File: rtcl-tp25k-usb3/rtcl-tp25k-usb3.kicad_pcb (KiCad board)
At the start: 4 copper layers, 80 x 35 mm, 109 parts, among them J1 ZX360D-B-10P(30), J10 SSQ-106-02-F-D-RA, J2 CF20221V0R0-NH, J3 DF40C(2.0)-60DS-0.4V(51), J4 DF40C(2.0)-60DS-0.4V(51), J5 JTAG, J6 Conn_01x02, J7 Conn_01x03, Q2 NTK3134NT1G, Q3 NTK3134NT1G, Q4 NTK3134NT1G, Q5 NTK3134NT1G, Q6 NTK3134NT1G, SW1 B3U-1100P, SW2 B3U-1100P, SW3 218-2LPSTR, SW4 B3U-1100P, U1 FT601Q, U2 TPD4E05U06DQA, U3 USBLC6-2P6, U4 TPS62826DMQR, U5 PCA9306DC, X1 ABM8-30.000MHZ-D1X-T

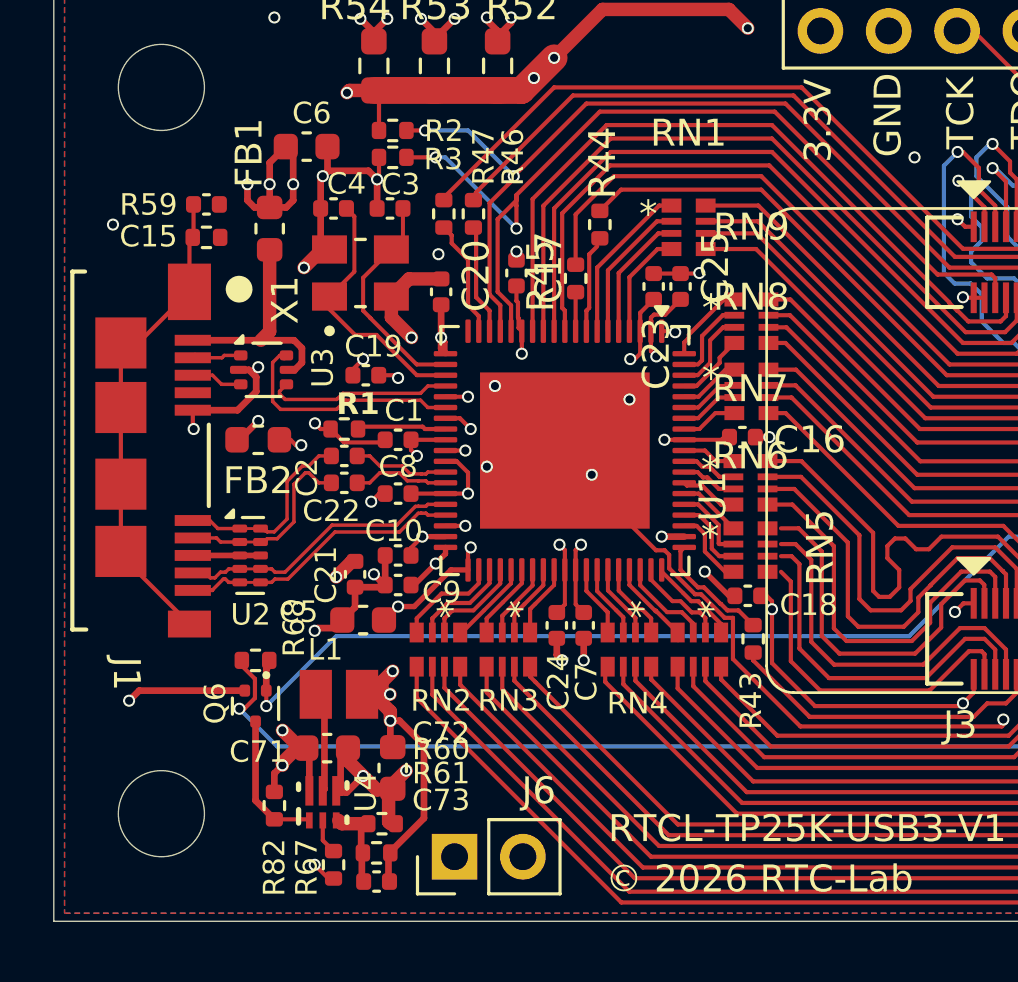
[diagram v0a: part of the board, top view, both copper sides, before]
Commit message: WIP
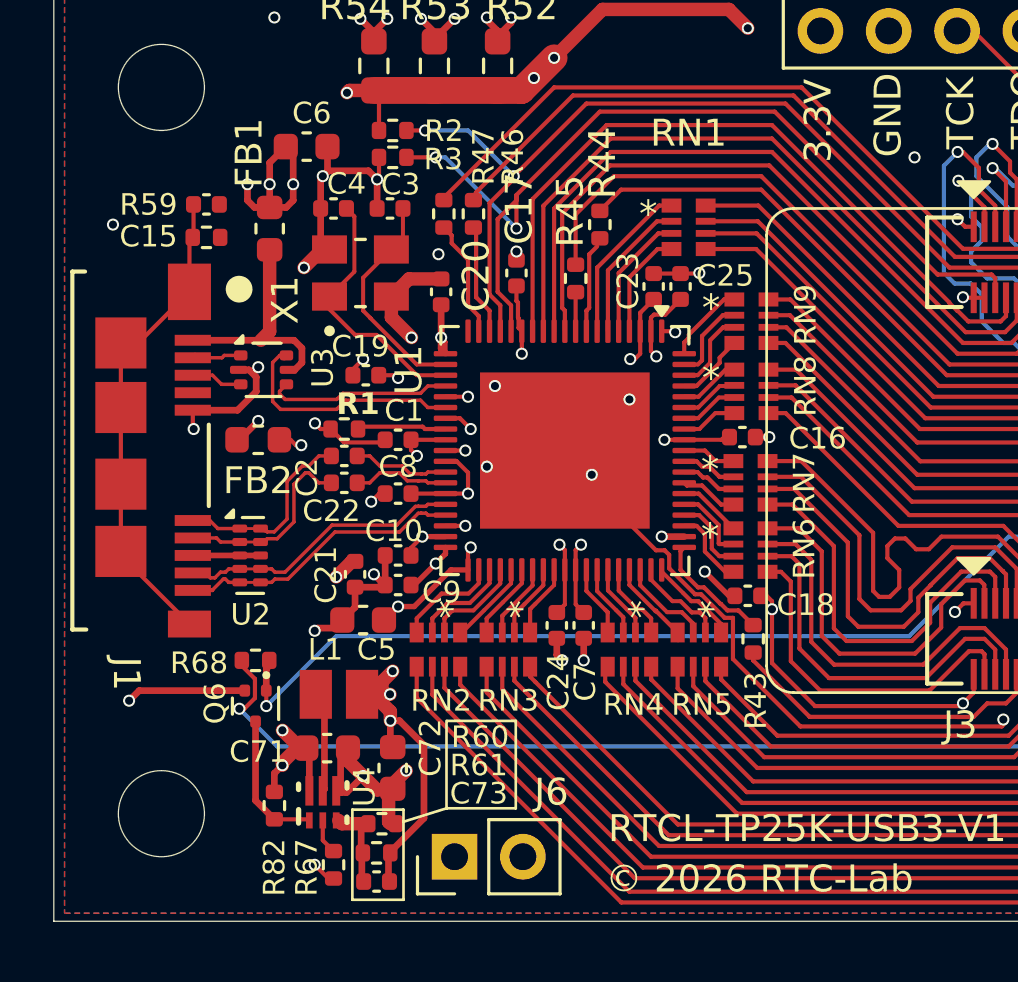
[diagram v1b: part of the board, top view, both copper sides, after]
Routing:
- net /L9_IOT31A_40P: track 13.7 -> 14.2 mm
- net /L5_IOT63A: track 13.8 -> 14.3 mm
- net /J5_IOT61B: track 13.4 -> 13.9 mm
- net /H5_IOT61A: track 12.5 -> 13.0 mm
